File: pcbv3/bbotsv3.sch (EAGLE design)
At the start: 15 parts

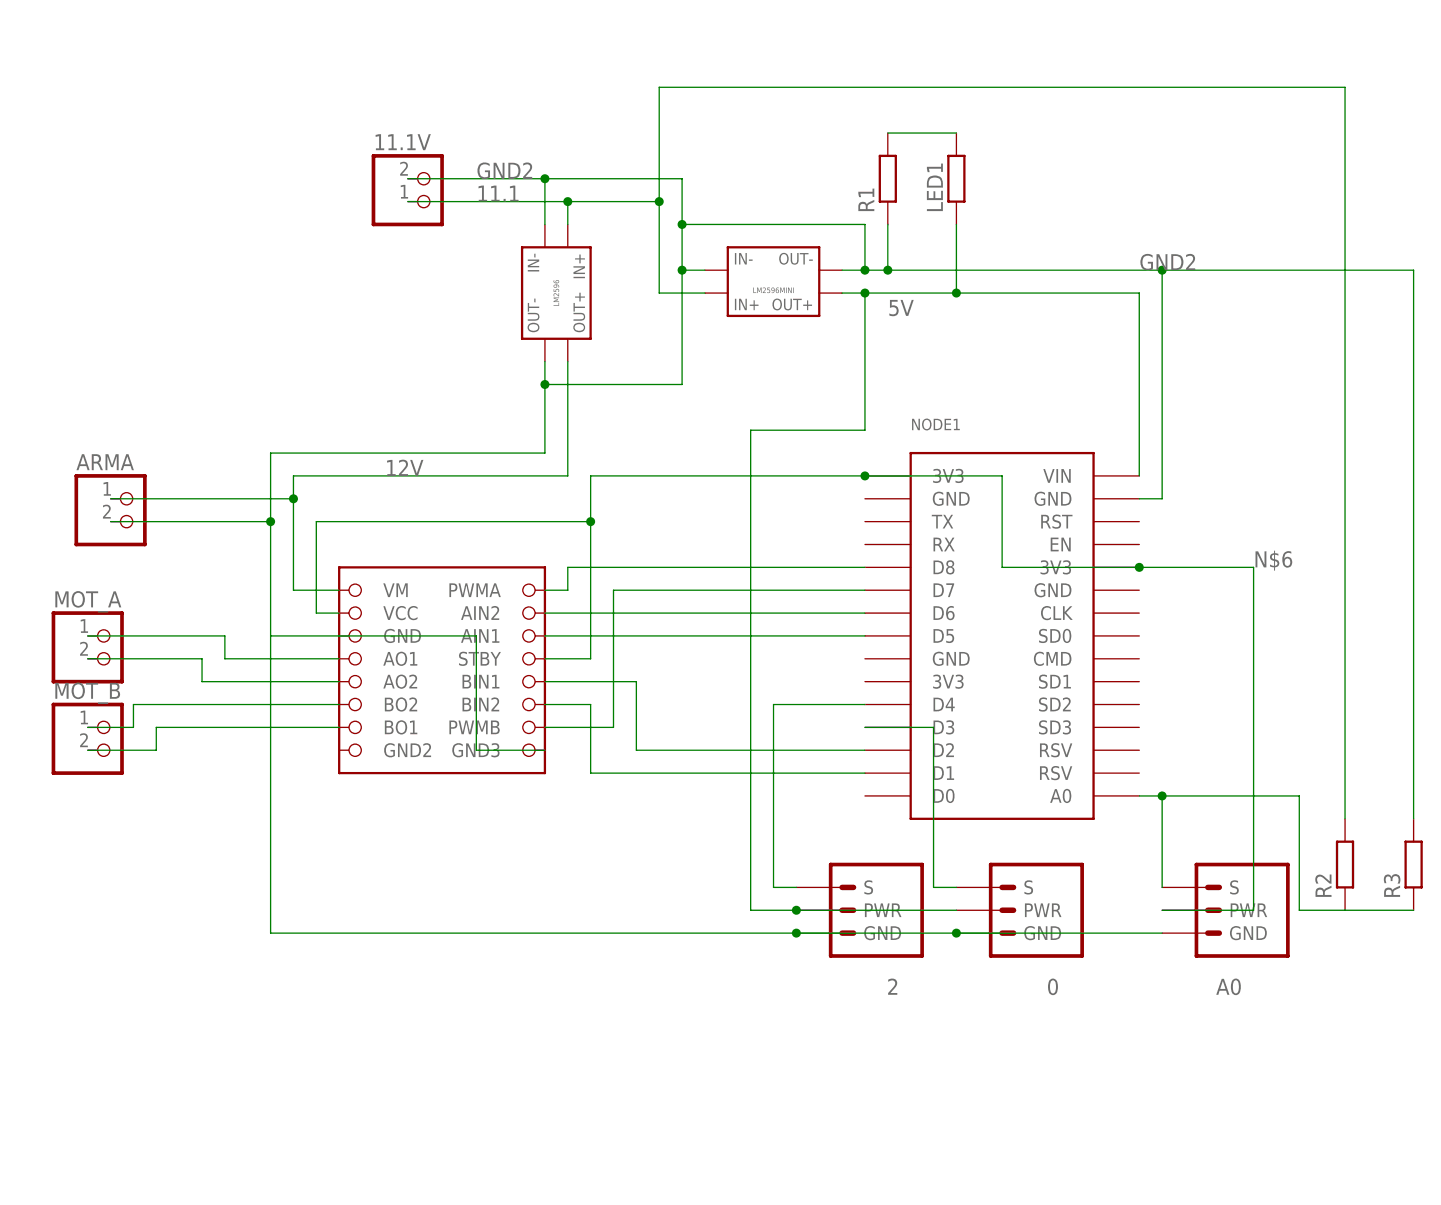
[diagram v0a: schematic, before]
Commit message: finish pcb, waiting review
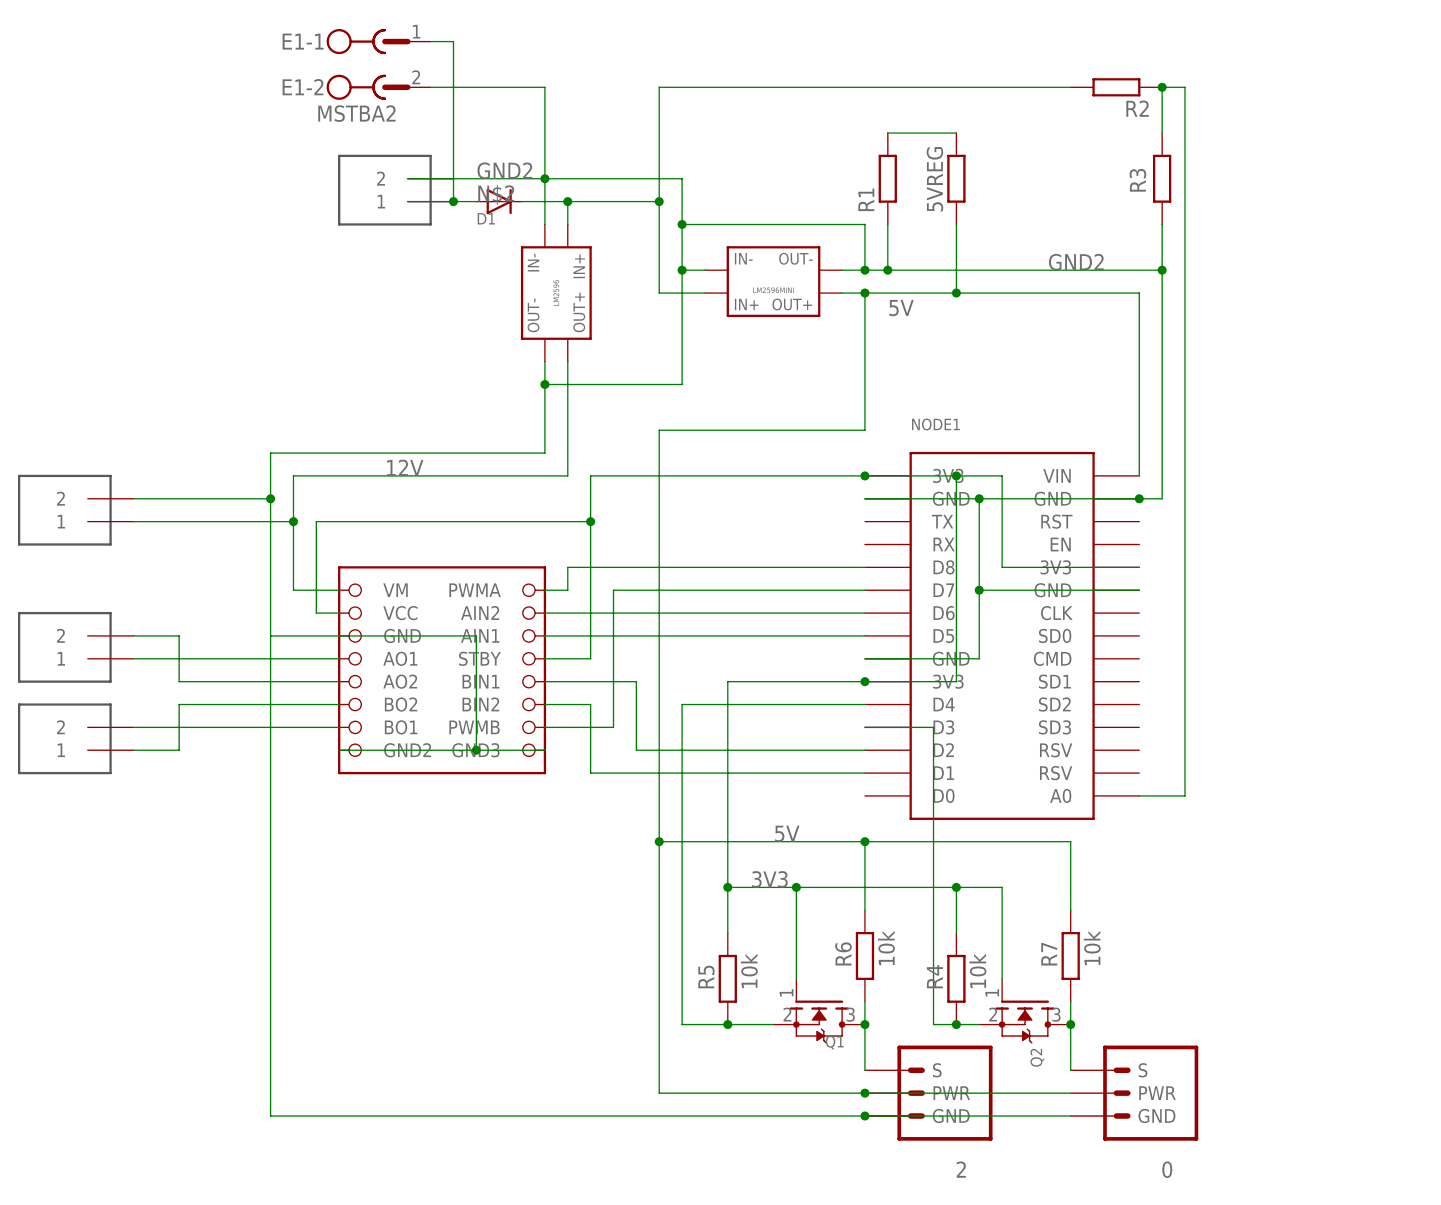
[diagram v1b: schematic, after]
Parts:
- removed 11.1V: (no value), adafruit:JST_2PIN-THM
- removed A0: 3.3, my-library:BB-PIN3BB-PIN3
- removed MOT_A, MOT_B: (no value), my-library:JST_2PIN
- added ARMA1, ARMA2, ARMA3: TERMINAL_2P, KF301-2P-Terminal:TERMINAL_2P
- added D1: (no value), adafruit:DIODEDO-1N4148
- added E1: MSTBA2, con-phoenix-508:MSTBA2
- added Q1, Q2: (no value), adafruit:MOSFET-NWAVE
- added R4, R5, R6, R7: 10k, my-library:BB-R1205
- ARMA: value (none) -> TERMINAL_2P; device my-library:JST_2PIN -> KF301-2P-Terminal:TERMINAL_2P
- R1: value BB-R1205 -> 100
- R2: value BB-R1205 -> 10k
- R3: value BB-R1205 -> 1k
- renumbered LED1 to 5VREG
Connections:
- removed net N$16: MOT_B.2, U$2.BO1
- new net 3V3: NODE1.3V3@1, NODE1.3V3@2, NODE1.3V3@3, Q1.G, Q2.G, R4.2, R5.2, U$2.STBY, U$2.VCC
- new net N$11: 2.S, Q1.D, R6.1
- new net N$19: NODE1.D4, Q1.S, R5.1
- new net N$2: ARMA3.1, D1.A, E1-1.1
- net 11.1: now also D1.C; no longer 11.1V.2
- net 5V: now also R6.2, R7.2
- net GND2: now also ARMA3.2, E1-2.1, NODE1.GND@1, NODE1.GND@2, NODE1.GND@3, U$2.GND2; no longer 11.1V.1, A0.GND
- net N$1: no longer A0.S
- net N$12: now also NODE1.D3, Q2.S, R4.1; no longer 2.S, NODE1.D4
- net N$13: now also ARMA1.2; no longer MOT_A.2
- net N$14: now also ARMA1.1; no longer MOT_A.1
- net N$15: now also ARMA2.2, U$2.BO1; no longer MOT_B.1, U$2.BO2
- net N$18: now also Q2.D, R7.1; no longer NODE1.D3
- net N$6: now also ARMA2.1, U$2.BO2; no longer A0.PWR, NODE1.3V3@1, NODE1.3V3@3, U$2.STBY, U$2.VCC
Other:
- moved on the sheet: 0, 2, R2, R3

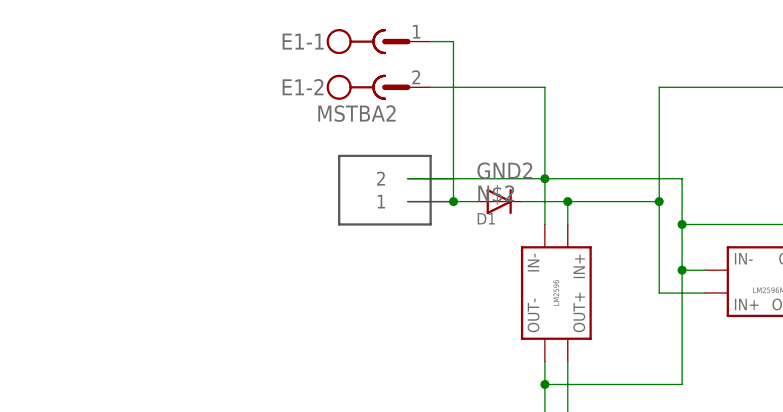
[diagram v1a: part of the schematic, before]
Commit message: ready to manufacture, review done
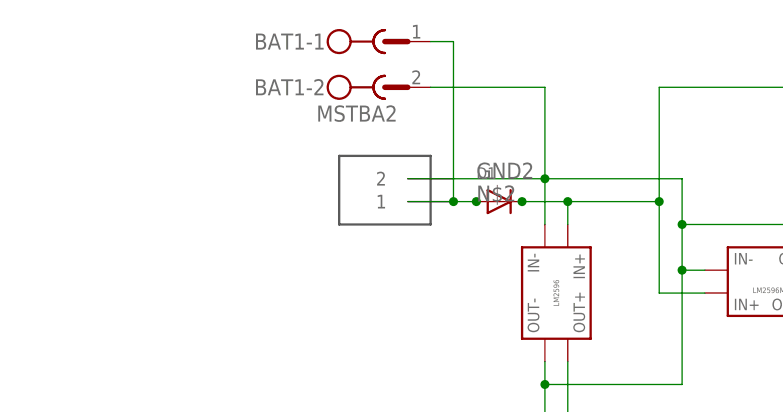
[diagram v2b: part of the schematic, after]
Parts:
- D1: device adafruit:DIODEDO-1N4148 -> my-library:DIODEDO-1N4148
- renumbered E1 to BAT1
